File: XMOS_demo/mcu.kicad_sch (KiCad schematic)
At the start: 40 parts, among them J1 XSYS2 DEBUG CONNECTOR, U1 U316-1024-QF60B, Y1 Crystal_24M

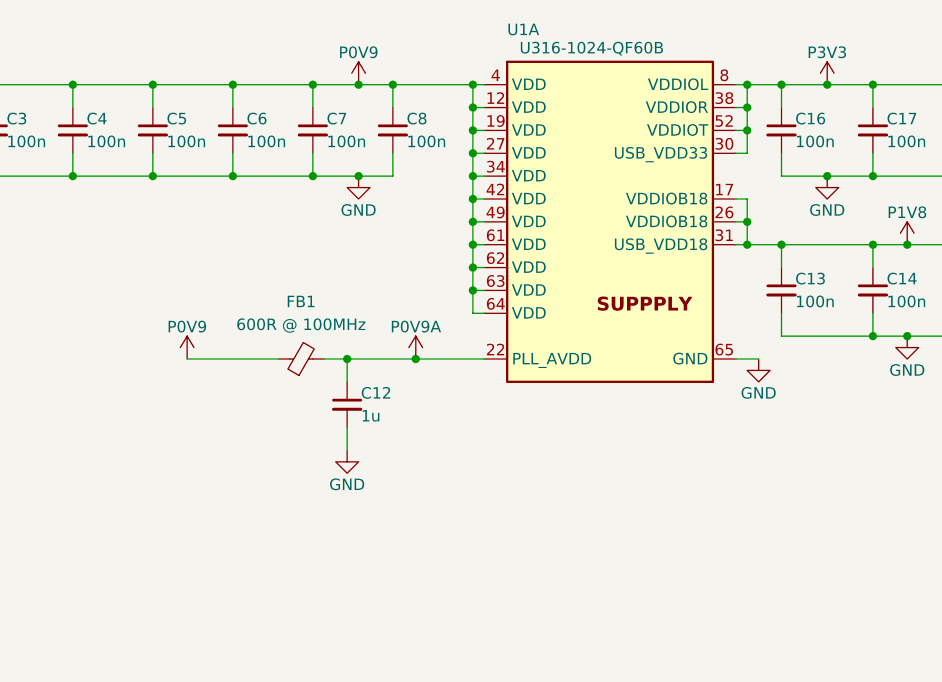
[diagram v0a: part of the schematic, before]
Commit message: Lots of sch work
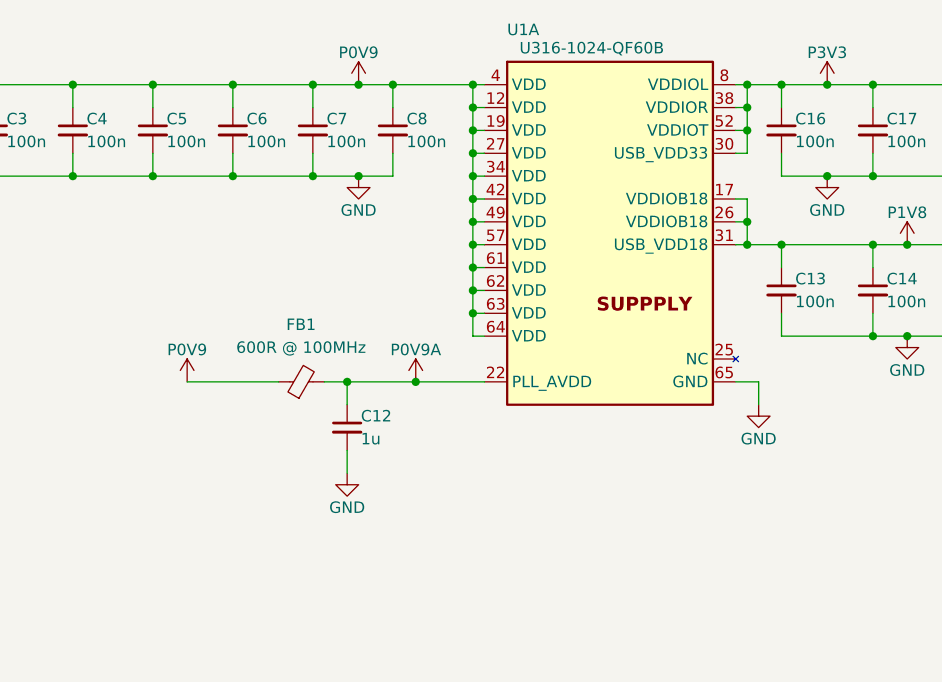
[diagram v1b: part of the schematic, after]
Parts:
- C1, C10, C13, C14, C15, C16, C17, C18, C19, C2, C3, C4, C5, C6, C7, C8, C9: Max Voltage 10V -> 16V
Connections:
- net P0V9: now also U1.57 (VDD)
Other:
- moved on the sheet: C12, FB1

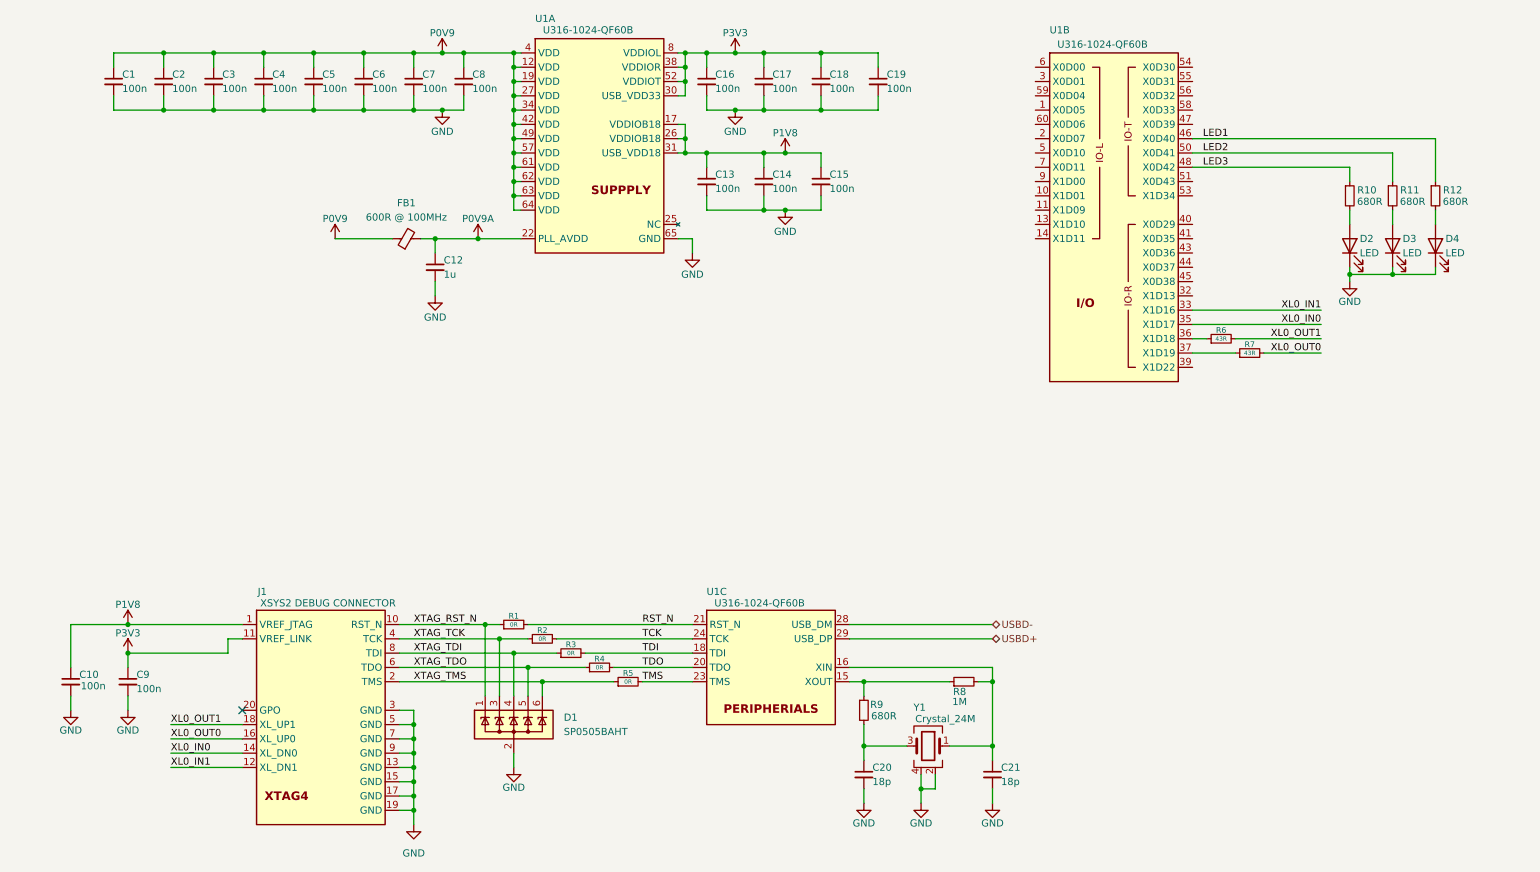
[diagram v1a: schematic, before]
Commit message: sch work, pcb import and initial board outline
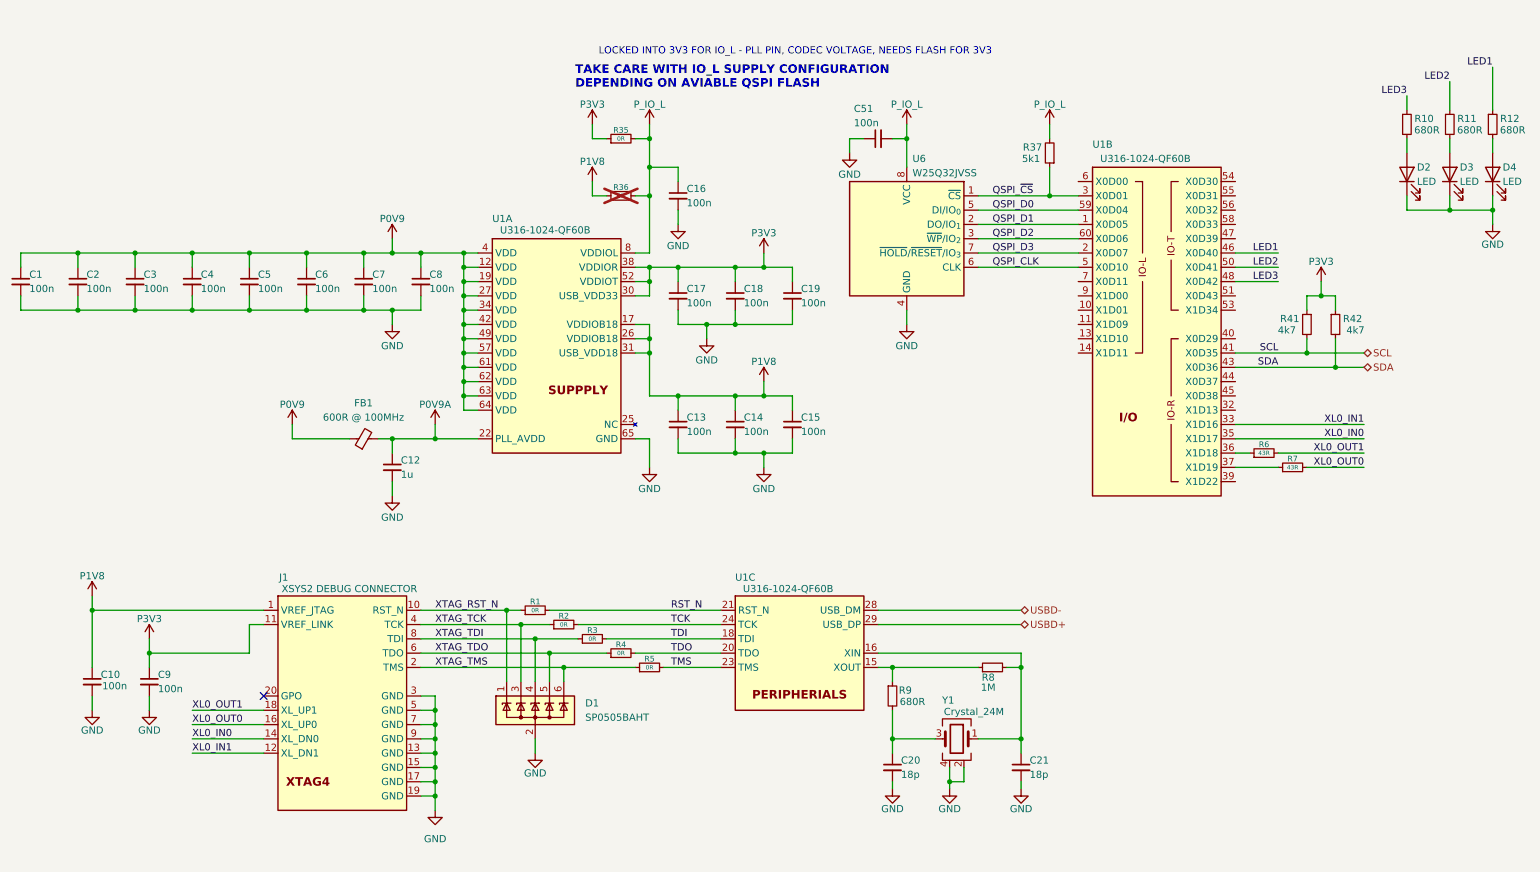
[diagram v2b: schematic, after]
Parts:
- added C51: 100n, Capacitor_SMD:C_0603_1608Metric, symbol Device:C_Small
- added R35, R36: 0R, Resistor_SMD:R_0603_1608Metric, symbol Device:R_Small
- added R37: 5k1, Resistor_SMD:R_0603_1608Metric, symbol Device:R_Small
- added R41, R42: 4k7, Resistor_SMD:R_0603_1608Metric, symbol Device:R_Small
- added U6: W25Q32JVSS, Package_SO:SOIC-8_5.3x5.3mm_P1.27mm, symbol Memory_Flash:W25Q32JVSS
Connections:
- net GND: now also C51.1, U6.4 (GND)
- net P1V8: now also R36.1
- net P3V3: now also R35.1, R41.1, R42.1; no longer C16.1, U1.8 (VDDIOL)
- net QSPI_D1: now reaches U1.1 (X0D05)
- net QSPI_D1: now also U6.2 (DO/IO_{1})
- net QSPI_D3: now reaches U1.2 (X0D07)
- net QSPI_D3: now also U6.7 (~{HOLD}/~{RESET}/IO_{3})
- net QSPI_~{CS}: now reaches U1.3 (X0D01)
- net QSPI_~{CS}: now also R37.1, U6.1 (~{CS})
- net SCL: now reaches U1.41 (X0D35)
- net SCL: now also R41.2
- net SDA: now reaches U1.43 (X0D36)
- net SDA: now also R42.2
- net QSPI_CLK: now reaches U1.5 (X0D10)
- net QSPI_CLK: now also U6.6 (CLK)
- net QSPI_D0: now reaches U1.59 (X0D04)
- net QSPI_D0: now also U6.5 (DI/IO_{0})
- net QSPI_D2: now reaches U1.60 (X0D06)
- net QSPI_D2: now also U6.3 (~{WP}/IO_{2})
- new net P_IO_L: C16.1, C51.2, R35.2, R36.2, R37.2, U1.8 (VDDIOL), U6.8 (VCC)
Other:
- note added: "LOCKED INTO 3V3 FOR IO_L - PLL PIN, CODEC VOLTAGE, NEEDS FLASH FOR 3V3"
- note added: "TAKE CARE WITH IO_L SUPPLY CONFIGURATION DEPENDING ON AVIABLE QSPI FLASH"
- moved on the sheet: C1, C10, C12, C13, C14, C15, C16, C17, C18, C19, C2, C20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
